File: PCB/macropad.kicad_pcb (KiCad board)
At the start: 2 copper layers, 81.7 x 61.9 mm, 11 parts, among them SW10 SW_Push, SW11 SW_Push, SW12 SW_Push, SW2 RotaryEncoder_Switch, SW3 SW_Push, SW4 SW_Push, SW5 SW_Push, SW6 SW_Push, SW7 SW_Push, SW8 SW_Push, U1 XIAO-RP2040-DIP

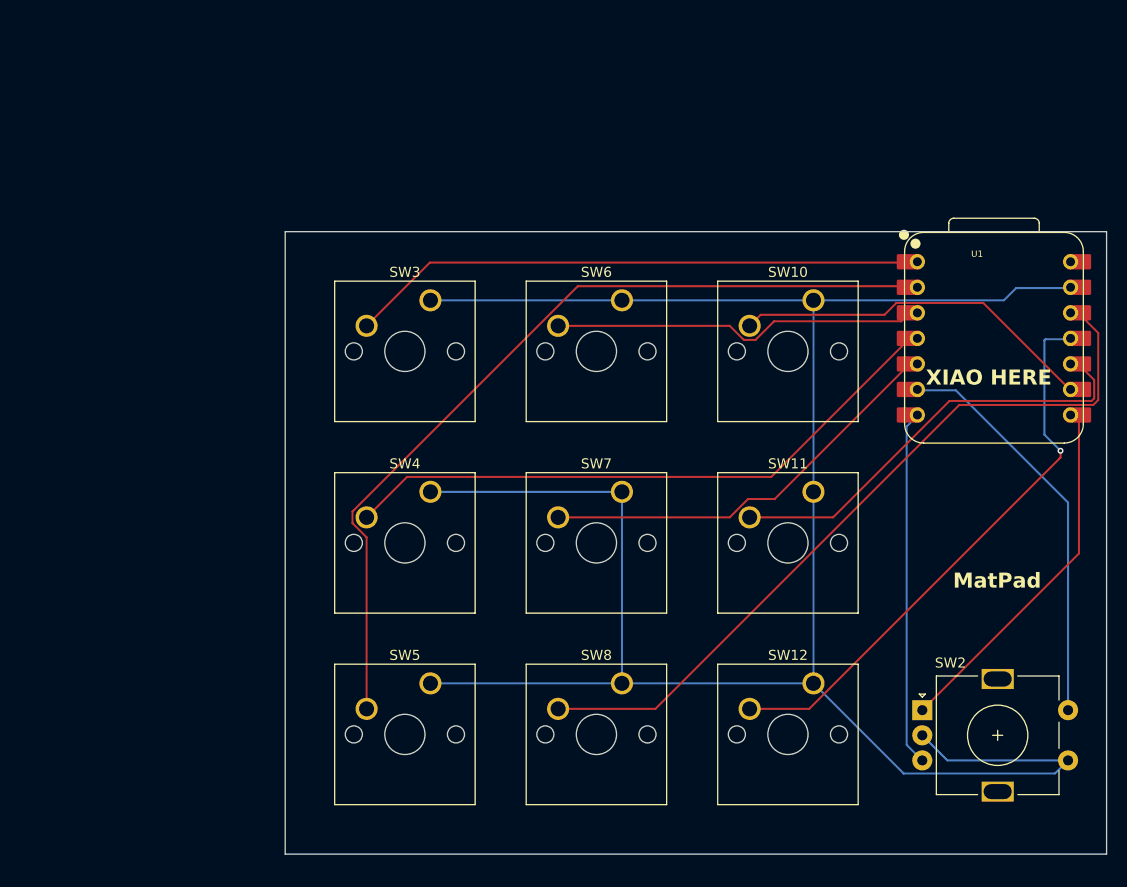
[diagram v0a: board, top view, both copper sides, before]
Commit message: Redesign
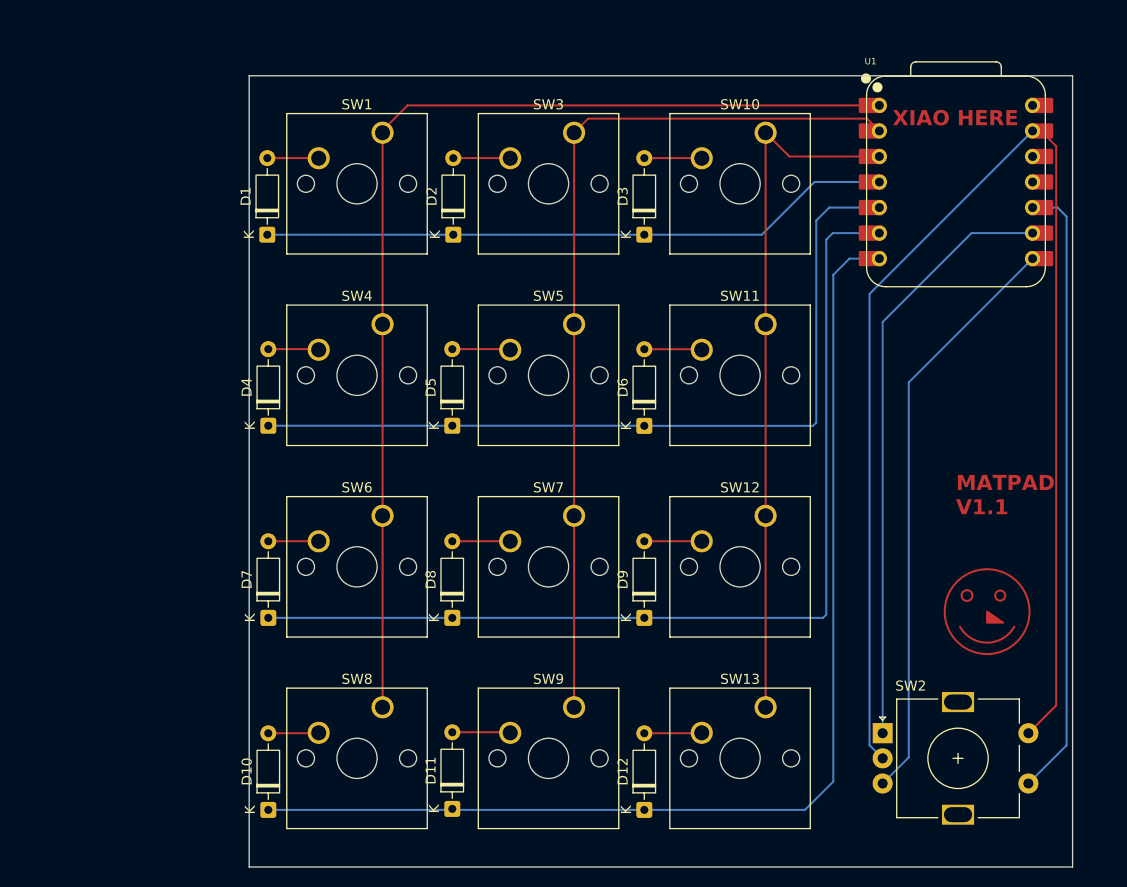
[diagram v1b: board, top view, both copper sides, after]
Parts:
- added D1: 1N4148, Diode_THT:D_DO-35_SOD27_P7.62mm_Horizontal, F.Cu at (114.9, 50.3)
- added D10: 1N4148, Diode_THT:D_DO-35_SOD27_P7.62mm_Horizontal, F.Cu at (115.0, 107.5)
- added D11: 1N4148, Diode_THT:D_DO-35_SOD27_P7.62mm_Horizontal, F.Cu at (133.3, 107.4)
- added D12: 1N4148, Diode_THT:D_DO-35_SOD27_P7.62mm_Horizontal, F.Cu at (152.4, 107.5)
- added D2: 1N4148, Diode_THT:D_DO-35_SOD27_P7.62mm_Horizontal, F.Cu at (133.4, 50.3)
- added D3: 1N4148, Diode_THT:D_DO-35_SOD27_P7.62mm_Horizontal, F.Cu at (152.4, 50.3)
- added D4: 1N4148, Diode_THT:D_DO-35_SOD27_P7.62mm_Horizontal, F.Cu at (115.0, 69.3)
- added D5: 1N4148, Diode_THT:D_DO-35_SOD27_P7.62mm_Horizontal, F.Cu at (133.3, 69.3)
- added D6: 1N4148, Diode_THT:D_DO-35_SOD27_P7.62mm_Horizontal, F.Cu at (152.4, 69.3)
- added D7: 1N4148, Diode_THT:D_DO-35_SOD27_P7.62mm_Horizontal, F.Cu at (115.0, 88.4)
- added D8: 1N4148, Diode_THT:D_DO-35_SOD27_P7.62mm_Horizontal, F.Cu at (133.3, 88.4)
- added D9: 1N4148, Diode_THT:D_DO-35_SOD27_P7.62mm_Horizontal, F.Cu at (152.4, 88.4)
- added SW1: SW_Push, Button_Switch_Keyboard:SW_Cherry_MX_1.00u_PCB, F.Cu at (126.4, 40.2)
- added SW13: SW_Push, Button_Switch_Keyboard:SW_Cherry_MX_1.00u_PCB, F.Cu at (164.5, 97.3)
- added SW9: SW_Push, Button_Switch_Keyboard:SW_Cherry_MX_1.00u_PCB, F.Cu at (145.4, 97.3)
- moved SW5 38.5 mm to (145.4, 59.2)
- moved SW6 32.0 mm to (126.4, 78.3)
- moved SW8 23.9 mm to (126.4, 97.3)
- moved SW3 22.0 mm to (145.4, 40.2)
- moved SW10 17.3 mm to (164.5, 40.2)
- moved SW12 17.3 mm to (164.5, 78.3)
- moved SW4 17.3 mm to (126.4, 59.2)
- moved SW11 17.3 mm to (164.5, 59.2)
- moved U1 16.0 mm to (183.4, 45.1)
- moved SW7 5.32 mm to (145.4, 78.3)
- moved SW2 4.56 mm to (176.1, 99.9)
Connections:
- SW10 pad 1: GND -> COL3
- SW10 pad 2: Net-(U1-GPIO2/SCK) -> Net-(D3-A)
- SW11 pad 1: GND -> COL3
- SW11 pad 2: Net-(U1-GPIO4/MISO) -> Net-(D6-A)
- SW12 pad 1: GND -> COL3
- SW12 pad 2: Net-(U1-GPIO3/MOSI) -> Net-(D9-A)
- SW2 pad A: Net-(U1-GPIO1/RX) -> Net-(U1-GPIO2/SCK)
- SW2 pad B: Net-(U1-GPIO0/TX) -> Net-(U1-GPIO1/RX)
- SW2 pad S1: GND -> Net-(U1-GPIO4/MISO)
- SW2 pad S2: Net-(U1-GPIO7/SCL) -> GND
- SW3 pad 1: GND -> COL2
- SW3 pad 2: Net-(U1-GPIO26/ADC0/A0) -> Net-(D2-A)
- SW4 pad 1: GND -> COL1
- SW4 pad 2: Net-(U1-GPIO29/ADC3/A3) -> Net-(D4-A)
- SW5 pad 1: GND -> COL2
- SW5 pad 2: Net-(U1-GPIO27/ADC1/A1) -> Net-(D5-A)
- SW6 pad 1: GND -> COL1
- SW6 pad 2: Net-(U1-GPIO28/ADC2/A2) -> Net-(D7-A)
- SW7 pad 1: GND -> COL2
- SW7 pad 2: Net-(U1-GPIO6/SDA) -> Net-(D8-A)
- SW8 pad 1: GND -> COL1
- SW8 pad 2: Net-(U1-3V3) -> Net-(D10-A)
- U1 pad 1: Net-(U1-GPIO26/ADC0/A0) -> COL1
- U1 pad 11: Net-(U1-GPIO3/MOSI) -> unconnected-(U1-GPIO3/MOSI-Pad11)
- U1 pad 12: Net-(U1-3V3) -> unconnected-(U1-3V3-Pad12)
- U1 pad 2: Net-(U1-GPIO27/ADC1/A1) -> COL2
- U1 pad 3: Net-(U1-GPIO28/ADC2/A2) -> COL3
- U1 pad 4: Net-(U1-GPIO29/ADC3/A3) -> ROW1
- U1 pad 5: Net-(U1-GPIO6/SDA) -> ROW2
- U1 pad 6: Net-(U1-GPIO7/SCL) -> ROW3
- U1 pad 7: Net-(U1-GPIO0/TX) -> ROW4
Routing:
- net ROW4: track 0.00 -> 113.0 mm
- net COL1: track 0.00 -> 108.0 mm
- net ROW3: track 0.00 -> 98.5 mm
- net GND: track 223.6 -> 131.3 mm
- net COL2: track 0.00 -> 88.6 mm
- net Net-(U1-GPIO27/ADC1/A1): track 84.9 -> 0.00 mm
- net ROW2: track 0.00 -> 81.6 mm
- net Net-(U1-3V3): track 75.8 -> 0.00 mm
- net COL3: track 0.00 -> 69.4 mm
- net ROW1: track 0.00 -> 63.1 mm
- net Net-(U1-GPIO29/ADC3/A3): track 61.3 -> 0.00 mm
- net Net-(U1-GPIO26/ADC0/A0): track 57.4 -> 0.00 mm
- net Net-(U1-GPIO3/MOSI): track 56.3 -> 0.00 mm, vias 1 -> 0
- net Net-(U1-GPIO6/SDA): track 41.2 -> 0.00 mm
- net Net-(U1-GPIO7/SCL): track 40.3 -> 0.00 mm
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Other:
- board size 81.7 x 61.9 mm -> 81.9 x 78.7 mm
- board text added: "MATPAD V1.1"
- board text removed: "MatPad"

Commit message: update
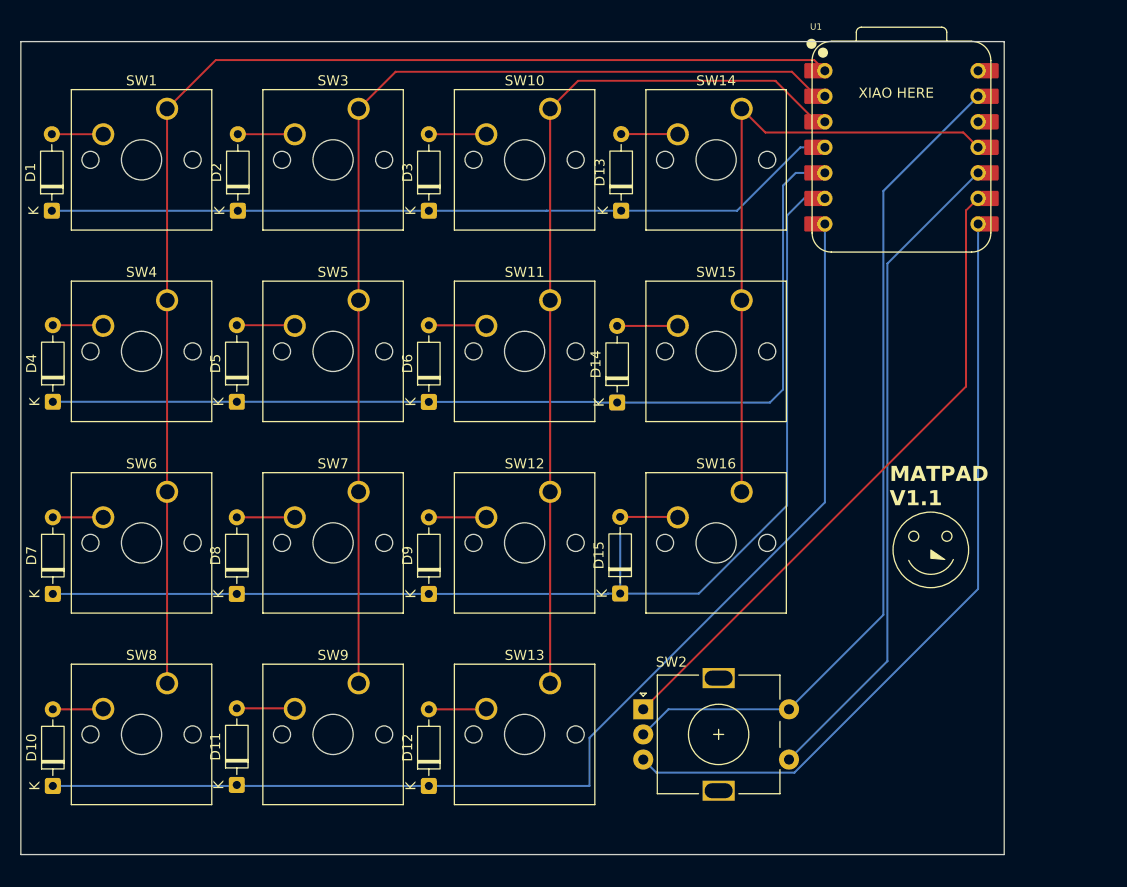
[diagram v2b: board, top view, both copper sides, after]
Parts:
- added D13: 1N4148, Diode_THT:D_DO-35_SOD27_P7.62mm_Horizontal, F.Cu at (150.1, 47.9)
- added D14: 1N4148, Diode_THT:D_DO-35_SOD27_P7.62mm_Horizontal, F.Cu at (149.7, 67.0)
- added D15: 1N4148, Diode_THT:D_DO-35_SOD27_P7.62mm_Horizontal, F.Cu at (150.0, 86.0)
- added SW14: SW_Push, Button_Switch_Keyboard:SW_Cherry_MX_1.00u_PCB, F.Cu at (162.1, 37.8)
- added SW15: SW_Push, Button_Switch_Keyboard:SW_Cherry_MX_1.00u_PCB, F.Cu at (162.1, 56.8)
- added SW16: SW_Push, Button_Switch_Keyboard:SW_Cherry_MX_1.00u_PCB, F.Cu at (162.1, 75.9)
- moved SW2 23.9 mm to (152.3, 97.5)
- moved D1 21.6 mm to (93.5, 47.9)
- moved D10 21.6 mm to (93.6, 105.1)
- moved D11 21.6 mm to (111.9, 105.0)
- moved D12 21.6 mm to (131.0, 105.1)
- moved D2 21.6 mm to (112.0, 47.9)
- moved D3 21.6 mm to (131.0, 47.9)
- moved D4 21.6 mm to (93.6, 66.9)
- moved D5 21.6 mm to (111.9, 66.9)
- moved D6 21.6 mm to (131.0, 66.9)
- moved D7 21.6 mm to (93.6, 86.0)
- moved D8 21.6 mm to (111.9, 86.0)
- moved D9 21.6 mm to (131.0, 86.0)
- moved SW10 21.6 mm to (143.0, 37.8)
- moved SW11 21.6 mm to (143.0, 56.8)
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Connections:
- U1 pad 11: unconnected-(U1-GPIO3/MOSI-Pad11) -> COL4
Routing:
- net COL4: track 0.00 -> 63.2 mm
- net GND: track 131.3 -> 84.3 mm
- net Net-(U1-GPIO1/RX): track 58.4 -> 77.7 mm
- net ROW3: track 98.5 -> 116.0 mm
- net COL1: track 108.0 -> 125.2 mm
- net COL3: track 69.4 -> 86.5 mm
- net COL2: track 88.6 -> 105.2 mm
- net ROW2: track 81.6 -> 98.2 mm
- net ROW1: track 63.1 -> 79.5 mm
- net Net-(D14-A): track 0.00 -> 6.04 mm
- net ROW4: track 113.0 -> 119.0 mm
- net Net-(D15-A): track 0.00 -> 5.75 mm
- net Net-(D13-A): track 0.00 -> 5.64 mm
- net Net-(U1-GPIO2/SCK): track 59.5 -> 64.6 mm
- net Net-(U1-GPIO4/MISO): track 61.7 -> 66.1 mm
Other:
- board size 81.9 x 78.7 mm -> 97.8 x 80.9 mm

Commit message: Add files via upload
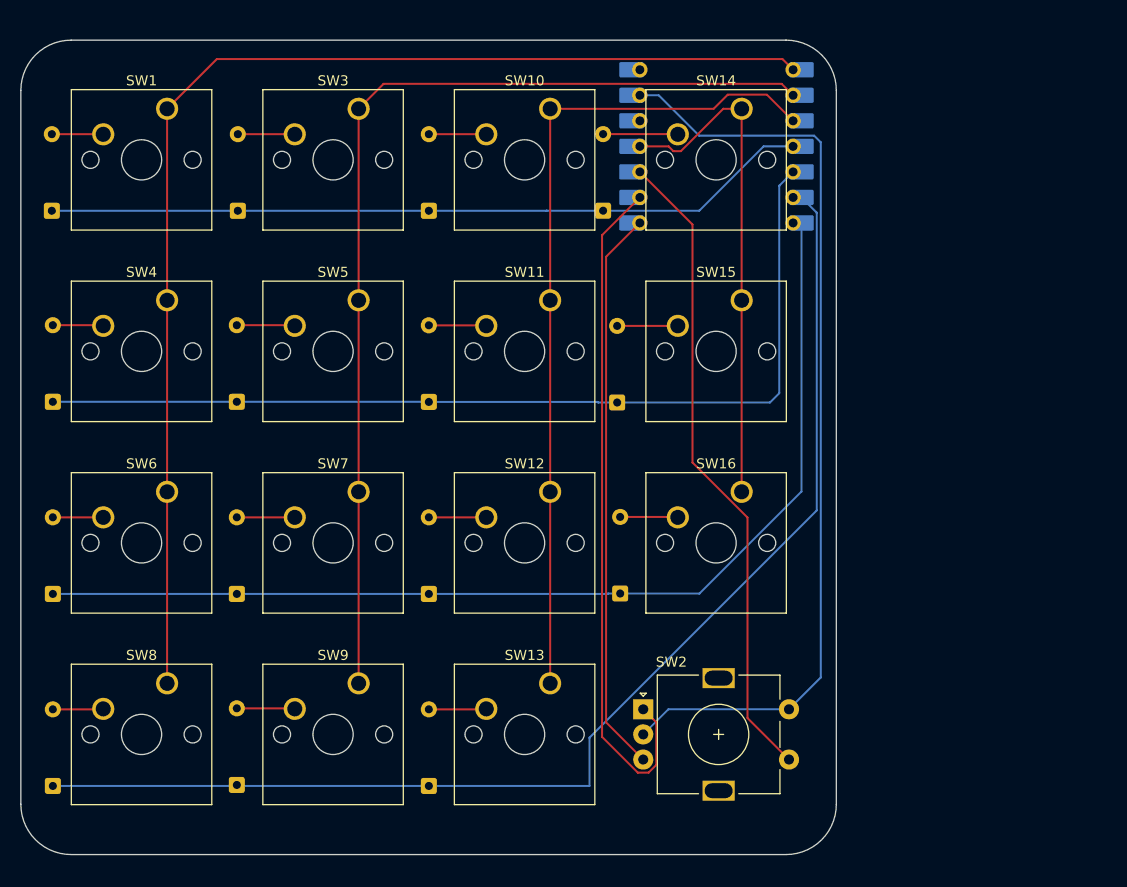
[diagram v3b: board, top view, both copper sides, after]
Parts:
- D1, D10, D11, D12, D13, D14, D15, D2, D3, D4, D5, D6, D7, D8, D9, U1: moved to B.Cu
- moved U1 18.4 mm to (159.6, 41.5), turned to 180 degrees
- moved D13 1.80 mm to (148.3, 47.9)
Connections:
- U1 pad 6: ROW3 -> ROW4
- U1 pad 7: ROW4 -> ROW3
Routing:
- net Net-(U1-GPIO1/RX): track 77.7 -> 56.3 mm
- net COL4: track 63.2 -> 50.2 mm
- net ROW3: track 116.0 -> 105.4 mm
- net GND: track 84.3 -> 93.2 mm
- net Net-(U1-GPIO2/SCK): track 64.6 -> 68.5 mm
- net COL3: track 86.5 -> 83.0 mm
- net COL2: track 105.2 -> 101.9 mm
- net COL1: track 125.2 -> 122.1 mm
- net ROW1: track 79.5 -> 76.4 mm
- net ROW4: track 119.0 -> 121.9 mm
- net ROW2: track 98.2 -> 95.3 mm
- net Net-(D13-A): track 5.64 -> 7.44 mm
- net Net-(U1-GPIO4/MISO): track 66.1 -> 64.6 mm
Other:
- board size 97.8 x 80.9 mm -> 81.1 x 81 mm
- board text removed: "MATPAD V1.1"
